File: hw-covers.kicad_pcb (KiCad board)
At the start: 2 copper layers, 135 x 75 mm, 110 parts, among them J1 Screw_Terminal_01x02, J2 Screw_Terminal_01x10, J3 Conn_01x04_Pin, J4 Conn_01x04_Pin, J5 Screw_Terminal_01x15, K1 JRC-21F(4100), K10 JRC-21F(4100), K2 JRC-21F(4100), K3 JRC-21F(4100), K4 JRC-21F(4100), K5 JRC-21F(4100), K6 JRC-21F(4100), K7 JRC-21F(4100), K8 JRC-21F(4100), K9 JRC-21F(4100), Q1 PMBT3904235, Q10 PMBT3904235, Q11 PMBT3904235, Q2 PMBT3904235, Q3 PMBT3904235, Q4 PMBT3904235, Q5 PMBT3904235, Q6 PMBT3904235, Q7 PMBT3904235, Q8 PMBT3904235, Q9 PMBT3904235, SW1 SW_Push, U2 NCP1117-3.3_SOT223, U3 HLK-2M05, U4 ESP32-S3-WROOM-1

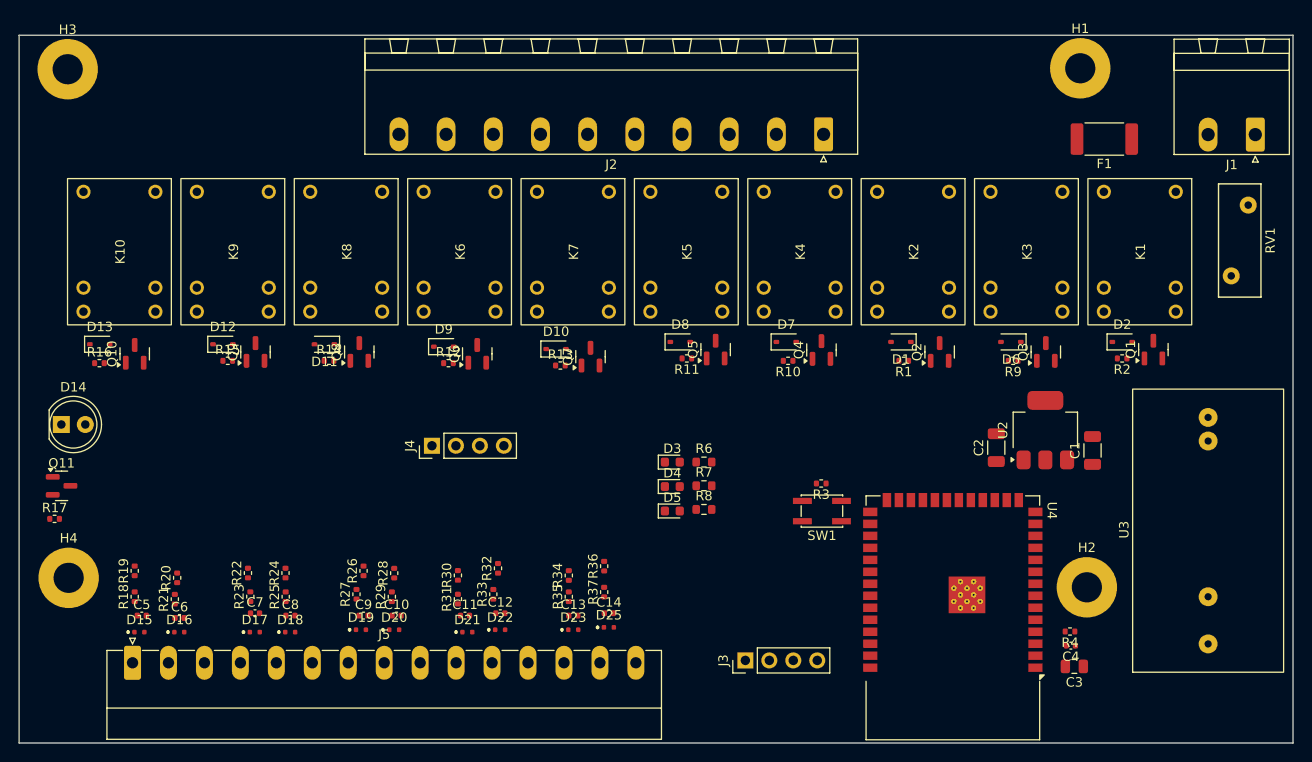
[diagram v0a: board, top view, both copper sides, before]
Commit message: Release 1.0
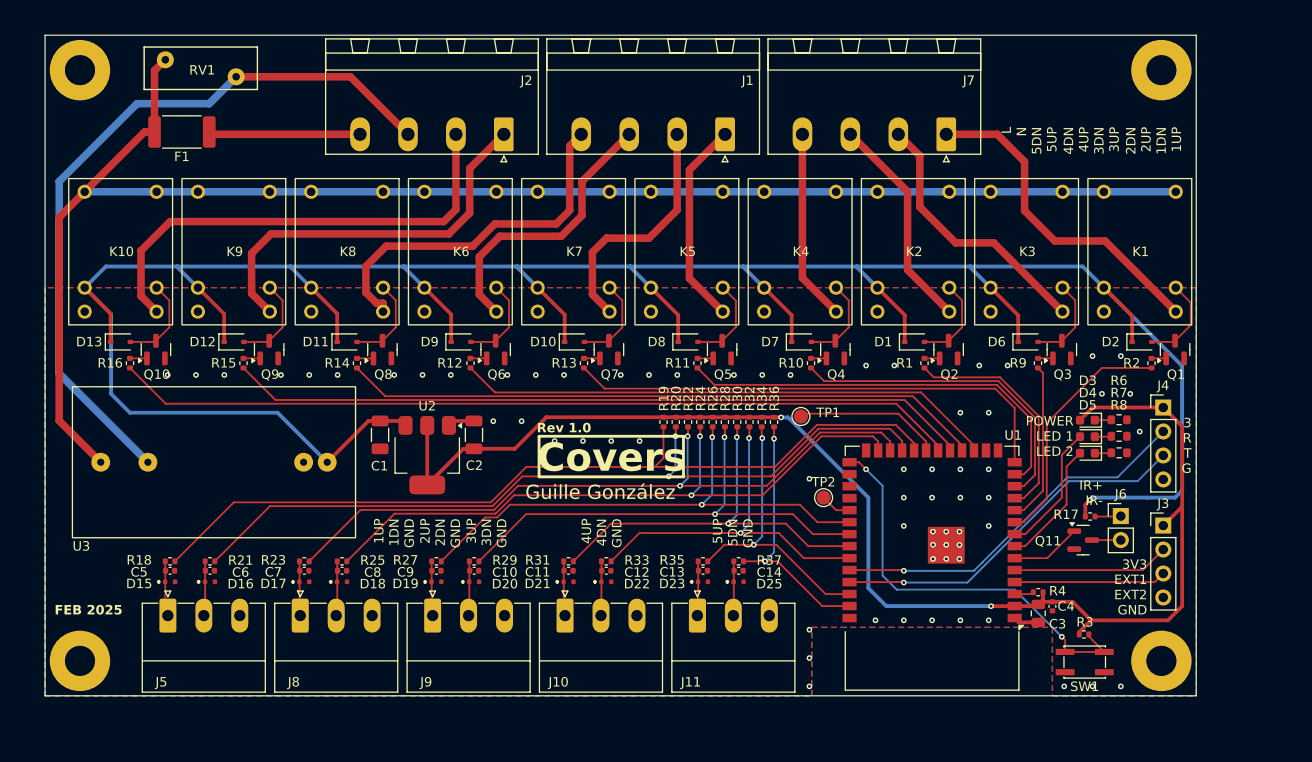
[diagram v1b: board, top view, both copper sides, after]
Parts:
- removed D14: LED, LED_THT:LED_D5.0mm
- removed U4: ESP32-S3-WROOM-1, RF_Module:ESP32-S3-WROOM-1
- added J10: Screw_Terminal_01x03, Connector_Phoenix_MC:PhoenixContact_MC_1,5_3-G-3.81_1x03_P3.81mm_Horizontal, F.Cu at (150.1, 113.5)
- added J11: Screw_Terminal_01x03, Connector_Phoenix_MC:PhoenixContact_MC_1,5_3-G-3.81_1x03_P3.81mm_Horizontal, F.Cu at (164.1, 113.5)
- added J6: Conn_01x02_Pin, Connector_PinHeader_2.54mm:PinHeader_1x02_P2.54mm_Vertical, F.Cu at (209.0, 103.0)
- added J7: Screw_Terminal_01x04, Connector_Phoenix_MSTB:PhoenixContact_MSTBA_2,5_4-G-5,08_1x04_P5.08mm_Horizontal, F.Cu at (190.5, 62.5)
- added J8: Screw_Terminal_01x03, Connector_Phoenix_MC:PhoenixContact_MC_1,5_3-G-3.81_1x03_P3.81mm_Horizontal, F.Cu at (122.0, 113.5)
- added J9: Screw_Terminal_01x03, Connector_Phoenix_MC:PhoenixContact_MC_1,5_3-G-3.81_1x03_P3.81mm_Horizontal, F.Cu at (136.1, 113.5)
- added TP1: TestPoint, TestPoint:TestPoint_Pad_D1.5mm, F.Cu at (175.1, 92.4)
- added TP2: TestPoint, TestPoint:TestPoint_Pad_D1.5mm, F.Cu at (177.5, 101.0)
- added U1: ESP32-S3-WROOM-1, guille-lib:ESP32-S3-WROOM-1, F.Cu at (189.0, 108.5)
- J1: value Screw_Terminal_01x02 -> Screw_Terminal_01x04; footprint Connector_Phoenix_MSTB:PhoenixContact_MSTBA_2,5_2-G_1x02_P5.00mm_Horizontal -> Connector_Phoenix_MSTB:PhoenixContact_MSTBA_2,5_4-G-5,08_1x04_P5.08mm_Horizontal
- J2: value Screw_Terminal_01x10 -> Screw_Terminal_01x04; footprint Connector_Phoenix_MSTB:PhoenixContact_MSTBA_2,5_10-G_1x10_P5.00mm_Horizontal -> Connector_Phoenix_MSTB:PhoenixContact_MSTBA_2,5_4-G-5,08_1x04_P5.08mm_Horizontal
- J5: value Screw_Terminal_01x15 -> Screw_Terminal_01x03; footprint Connector_Phoenix_MC:PhoenixContact_MC_1,5_15-G-3.81_1x15_P3.81mm_Horizontal -> Connector_Phoenix_MC:PhoenixContact_MC_1,5_3-G-3.81_1x03_P3.81mm_Horizontal
- moved RV1 115.2 mm to (107.8, 54.6), turned to 0 degrees
- moved R17 109.7 mm to (205.8, 103.0)
- moved Q11 108.4 mm to (205.0, 105.5)
- moved U3 105.5 mm to (113.0, 97.2), turned to 0 degrees
- moved F1 97.8 mm to (109.5, 62.2)
- moved J4 77.6 mm to (213.5, 91.5), turned to 0 degrees
- moved C1 75.5 mm to (130.5, 94.3), turned to -90 degrees
- moved U2 65.6 mm to (135.5, 96.5), turned to -90 degrees
- moved R19 58.2 mm to (160.5, 93.0)
- moved J1 56.2 mm to (167.1, 62.5)
- moved C2 55.4 mm to (140.4, 94.3)
- moved R20 55.4 mm to (161.8, 93.0)
- moved R22 49.3 mm to (163.1, 93.0)
- moved R24 46.8 mm to (164.4, 93.0)
- moved J3 46.5 mm to (213.5, 104.0), turned to 0 degrees
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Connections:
- J1 pad 1: /N -> /OUT3_UP
- J1 pad 2: /L -> /OUT3_DOWN
- J2 pad 1: /OUT1_UP -> /OUT5_UP
- J2 pad 2: /OUT1_DOWN -> /OUT5_DOWN
- J2 pad 3: /OUT2_UP -> /N
- J2 pad 4: /OUT2_DOWN -> /L
- J4 pad 2: /ESP_TX -> /ESP_RX
- J4 pad 3: /ESP_RX -> /ESP_TX
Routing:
- net +5V: track 0.00 -> 290.1 mm, vias 0 -> 1
- net /LF: track 0.00 -> 165.4 mm
- net +3V3: track 0.00 -> 142.4 mm, vias 0 -> 2
- net /1IN1: track 0.00 -> 90.5 mm
- net /5OUT2: track 0.00 -> 89.6 mm
- net /1IN2: track 0.00 -> 85.8 mm, vias 0 -> 2
- net /5OUT1: track 0.00 -> 78.8 mm
- net /N: track 0.00 -> 77.7 mm
- net /2IN1: track 0.00 -> 75.2 mm, vias 0 -> 2
- net /2IN2: track 0.00 -> 70.6 mm, vias 0 -> 2
- net /4OUT2: track 0.00 -> 68.1 mm
- net /4OUT1: track 0.00 -> 57.3 mm
- net /3IN1: track 0.00 -> 55.2 mm, vias 0 -> 2
- net /3OUT2: track 0.00 -> 53.1 mm
- net /3IN2: track 0.00 -> 51.9 mm, vias 0 -> 2
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- added copper zone on B.Cu, net GND
- added copper zone on F.Cu, net GND
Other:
- board size 135 x 75 mm -> 122 x 70 mm
- board text added: "1UP 1DN 2UP 2DN"
- board text added: "1UP 1DN GND"
- board text added: "2DN 2UP 1DN 1UP"
- board text added: "2UP 2DN GND"
- board text added: "3 R T G"
- board text added: "3UP 3DN 4UP 4DN"
- board text added: "3UP 3DN GND"
- board text added: "3V3 EXT1 EXT2 GND"
- board text added: "3V3 RX TX GND"
- board text added: "4DN 4UP 3DN 3UP"
- board text added: "4UP 4DN GND"
- board text added: "5UP 5DN GND"
- board text added: "5UP 5DN N L"
- board text added: "Covers"
- board text added: "FEB 2025"
- board text added: "GND 1DN 1UP"
- board text added: "GND 2DN 2UP"
- board text added: "GND 3DN 3UP"
- board text added: "GND 4DN 4UP"
- board text added: "GND 5DN 5UP"
- board text added: "Guille González"
- board text added: "IR+ IR-"
- board text added: "L N 5DN 5UP"
- board text added: "POWER LED 1 LED 2"
- board text added: "Rev 1.0"
